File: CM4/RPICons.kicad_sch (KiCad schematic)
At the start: 6 parts, among them U1 Compute_Module_4_Connectors

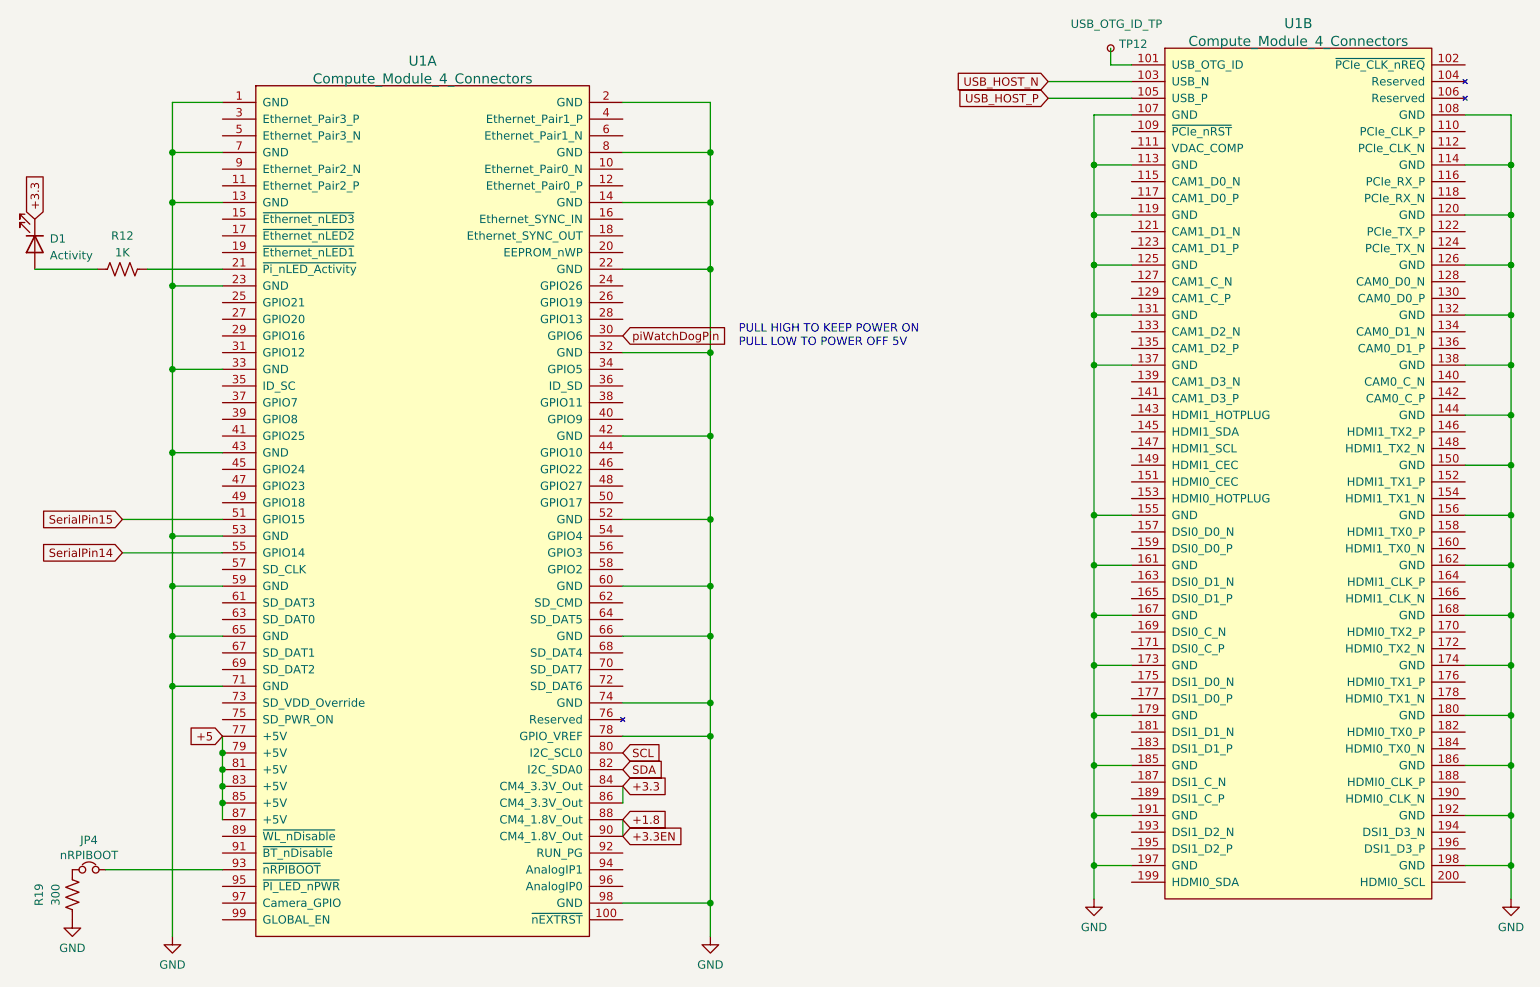
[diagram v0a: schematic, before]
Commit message: Finally Added the display!!!!
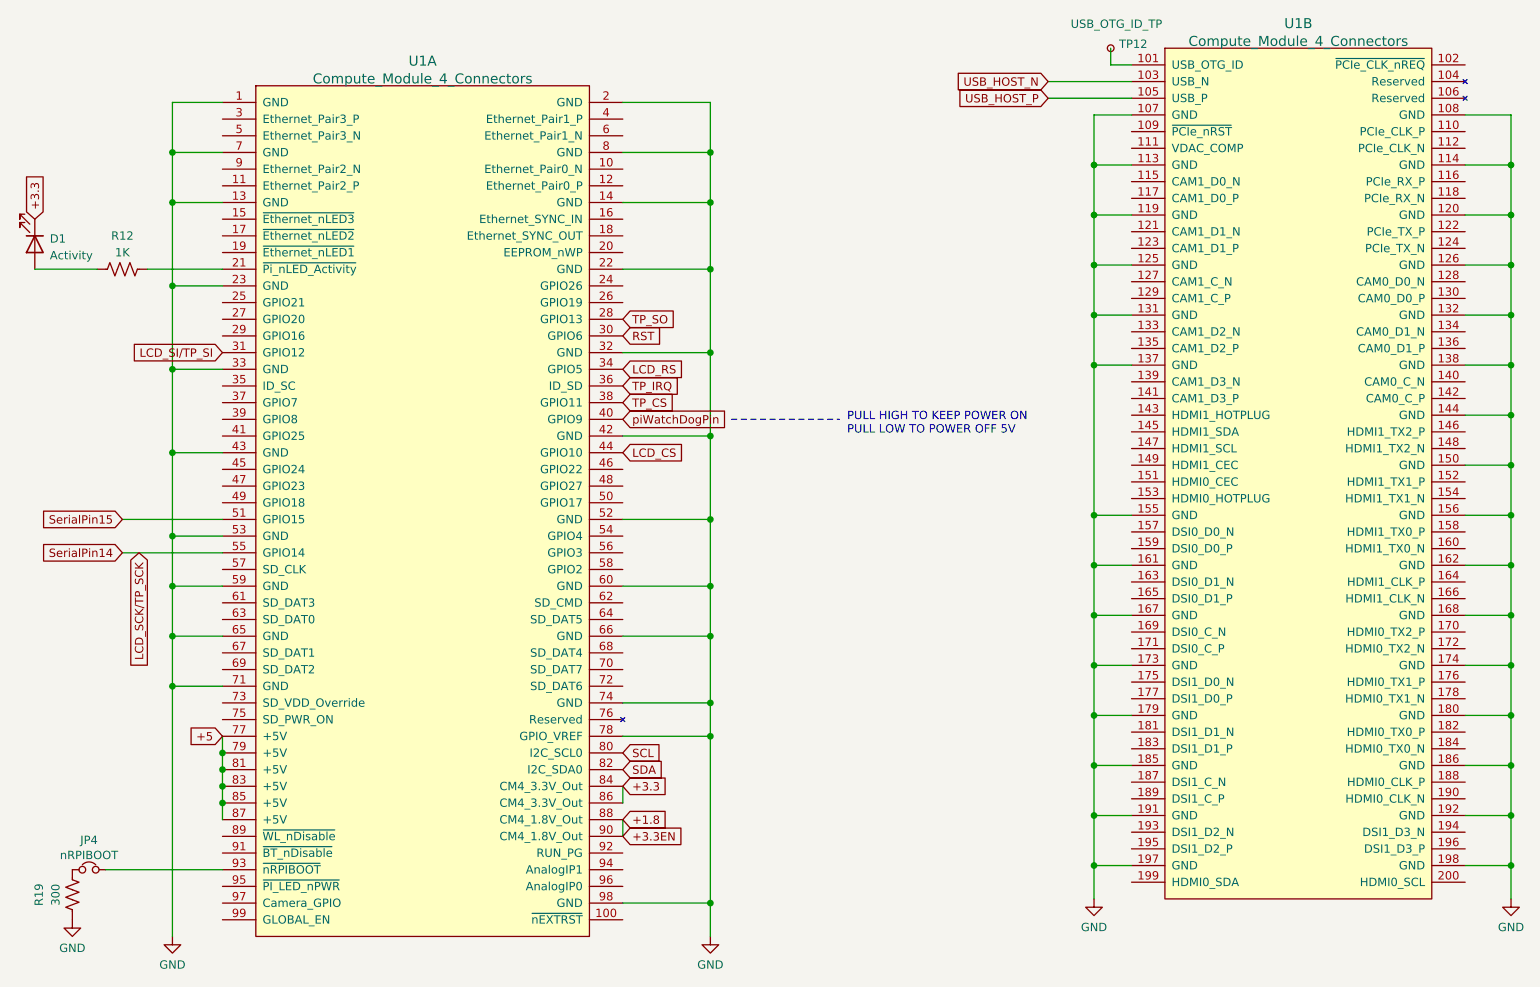
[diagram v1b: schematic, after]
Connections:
- net piWatchDogPin: now also U1.40 (GPIO9); no longer U1.30 (GPIO6)
- net TP_SO: now reaches U1.28 (GPIO13)
- net LCD_SI/TP_SI: now reaches U1.31 (GPIO12)
- net LCD_RS: now reaches U1.34 (GPIO5)
- net TP_IRQ: now reaches U1.36 (ID_SD)
- net TP_CS: now reaches U1.38 (GPIO11)
- net LCD_CS: now reaches U1.44 (GPIO10)
- net SerialPin14 renamed LCD_SCK/TP_SCK
- new net RST: U1.30 (GPIO6)
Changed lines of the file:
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@@
     (stroke (width 0) (type solid) (color 0 0 0 0))
   )
+  (polyline (pts (xy 128.905 81.28) (xy 145.415 81.28))
+    (stroke (width 0) (type dash) (color 0 0 0 0))
+  )
   (text "PULL HIGH TO KEEP POWER ON\nPULL LOW TO POWER OFF 5V"
-    (at 130.048 70.358 0)
+    (at 146.558 83.693 0)
     (effects (font (size 1.27 1.27)) (justify left bottom))
   )
@@
     )
   )
+  (global_label "LCD_SCK{slash}TP_SCK" (shape input) (at 38.735 101.6 270)
+    (effects (font (size 1.27 1.27)) (justify right))
+    (property "Intersheet References" "${INTERSHEET_REFS}" (id 0) (at 38.6556 120.5836 90)
+      (effects (font (size 1.27 1.27)) (justify right) hide)
+    )
+  )
+  (global_label "LCD_SI{slash}TP_SI" (shape input) (at 51.435 71.12 180)
+    (effects (font (size 1.27 1.27)) (justify right))
+    (property "Intersheet References" "${INTERSHEET_REFS}" (id 0) (at 36.3219 71.0406 0)
+      (effects (font (size 1.27 1.27)) (justify right) hide)
+    )
+  )
   (global_label "+5" (shape input) (at 51.435 129.54 180)
     (effects (font (size 1.27 1.27)) (justify right))
@@
     )
   )
-  (global_label "piWatchDogPin" (shape input) (at 112.395 68.58 0)
+  (global_label "TP_SO" (shape input) (at 112.395 66.04 0)
     (effects (font (size 1.27 1.27)) (justify left))
-    (property "Intersheet References" "${INTERSHEET_REFS}" (id 0) (at 128.7176 68.6594 0)
+    (property "Intersheet References" "${INTERSHEET_REFS}" (id 0) (at 120.5533 65.9606 0)
       (effects (font (size 1.27 1.27)) (justify left) hide)
     )
+  )
+  (global_label "RST" (shape input) (at 112.395 68.58 0)
+    (effects (font (size 1.27 1.27)) (justify left))
+    (property "Intersheet References" "${INTERSHEET_REFS}" (id 0) (at 118.2552 68.5006 0)
+      (effects (font (size 1.27 1.27)) (justify left) hide)
+    )
+  )
+  (global_label "LCD_RS" (shape input) (at 112.395 73.66 0)
+    (effects (font (size 1.27 1.27)) (justify left))
+    (property "Intersheet References" "${INTERSHEET_REFS}" (id 0) (at 121.8233 73.5806 0)
+      (effects (font (size 1.27 1.27)) (justify left) hide)
+    )
+  )
+  (global_label "TP_IRQ" (shape input) (at 112.395 76.2 0)
+    (effects (font (size 1.27 1.27)) (justify left))
+    (property "Intersheet References" "${INTERSHEET_REFS}" (id 0) (at 121.2186 76.1206 0)
+      (effects (font (size 1.27 1.27)) (justify left) hide)
+    )
+  )
+  (global_label "TP_CS" (shape input) (at 112.395 78.74 0)
+    (effects (font (size 1.27 1.27)) (justify left))
+    (property "Intersheet References" "${INTERSHEET_REFS}" (id 0) (at 120.4929 78.6606 0)
+      (effects (font (size 1.27 1.27)) (justify left) hide)
+    )
+  )
+  (global_label "piWatchDogPin" (shape input) (at 112.395 81.28 0)
+    (effects (font (size 1.27 1.27)) (justify left))
+    (property "Intersheet References" "${INTERSHEET_REFS}" (id 0) (at 128.7176 81.3594 0)
+      (effects (font (size 1.27 1.27)) (justify left) hide)
+    )
+  )
+  (global_label "LCD_CS" (shape input) (at 112.395 86.36 0)
+    (effects (font (size 1.27 1.27)) (justify left))
+    (property "Intersheet References" "${INTERSHEET_REFS}" (id 0) (at 121.8233 86.2806 0)
+      (effects (font (size 1.27 1.27)) (justify left) hide)
+    )
